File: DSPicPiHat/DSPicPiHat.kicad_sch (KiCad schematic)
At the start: 85 parts, among them J1 Conn_01x09_Female, J2 Conn_01x04_Female, J4 Conn_PIC_ICSP_ICD, J5 USB_C_Receptacle_USB2.0, J6 PowerInput, J8 RasPiHeaders, SW1 POWER_Select, SW2 SW_DIP_x08, U1 DSPIC33CH512MP508T-I_PT, U10 DF5A6.2CJE_LM, U11 FT230XS, U12 NCP1117-3.3_SOT223, U3 DF5A6.2CJE_LM, U4 DF5A6.2CJE_LM, U6 DF5A6.2CJE_LM, U7 DF5A6.2CJE_LM, U9 DF5A6.2CJE_LM, Y1 16MHz

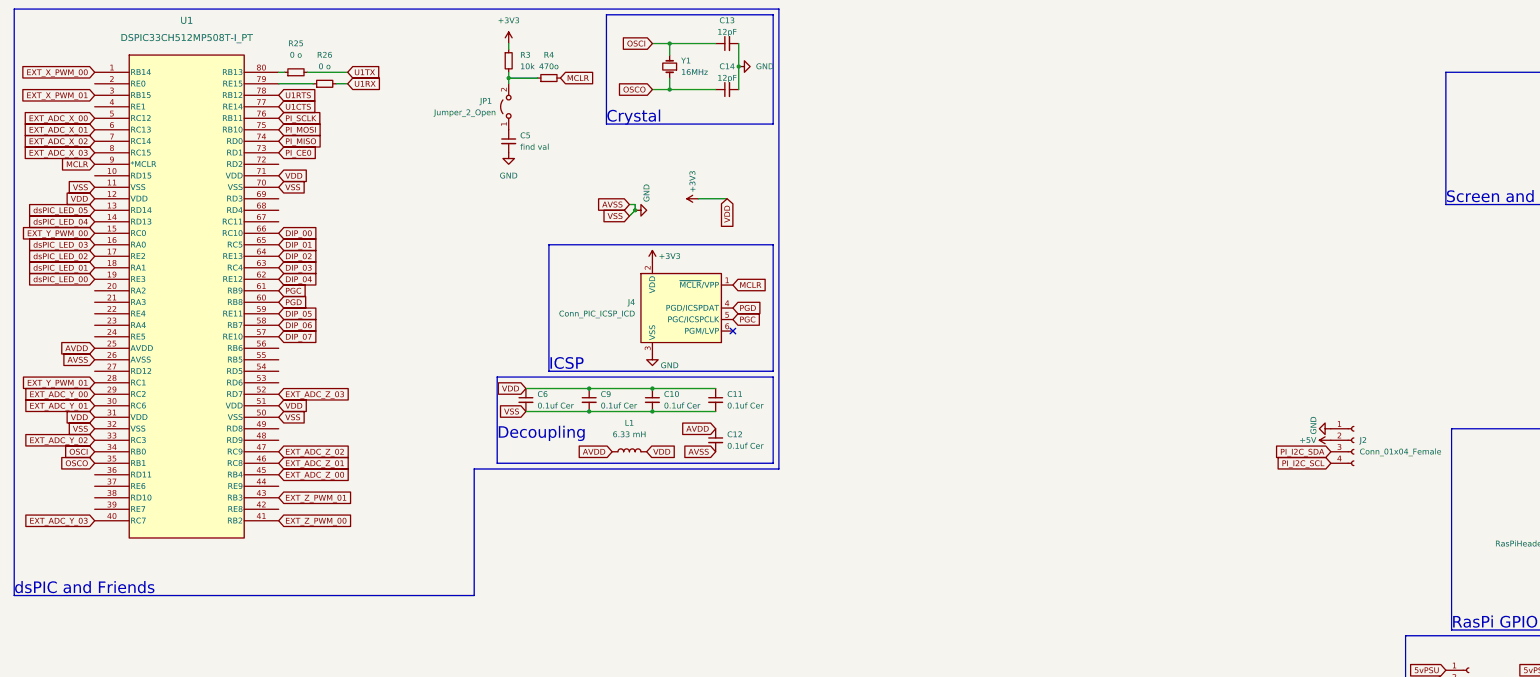
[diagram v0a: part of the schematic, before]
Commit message: organized schem
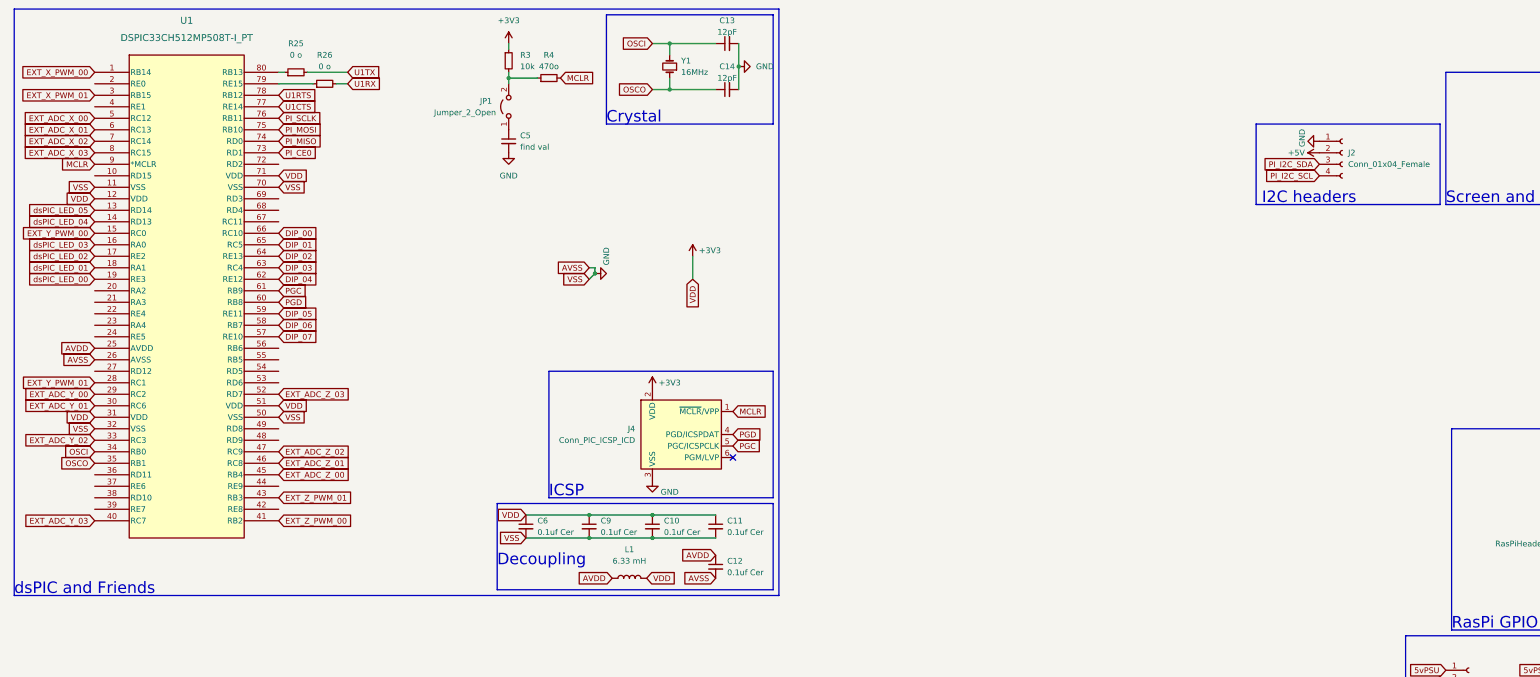
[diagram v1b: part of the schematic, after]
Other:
- note added: "I2C headers"
- moved on the sheet: C10, C11, C12, C6, C9, J2, J4, L1
